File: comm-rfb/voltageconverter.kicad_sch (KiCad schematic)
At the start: 12 parts, among them Q1 Q_PMOS_DGS, U3 BU33SA5WGWZ-E2-qsat-symb

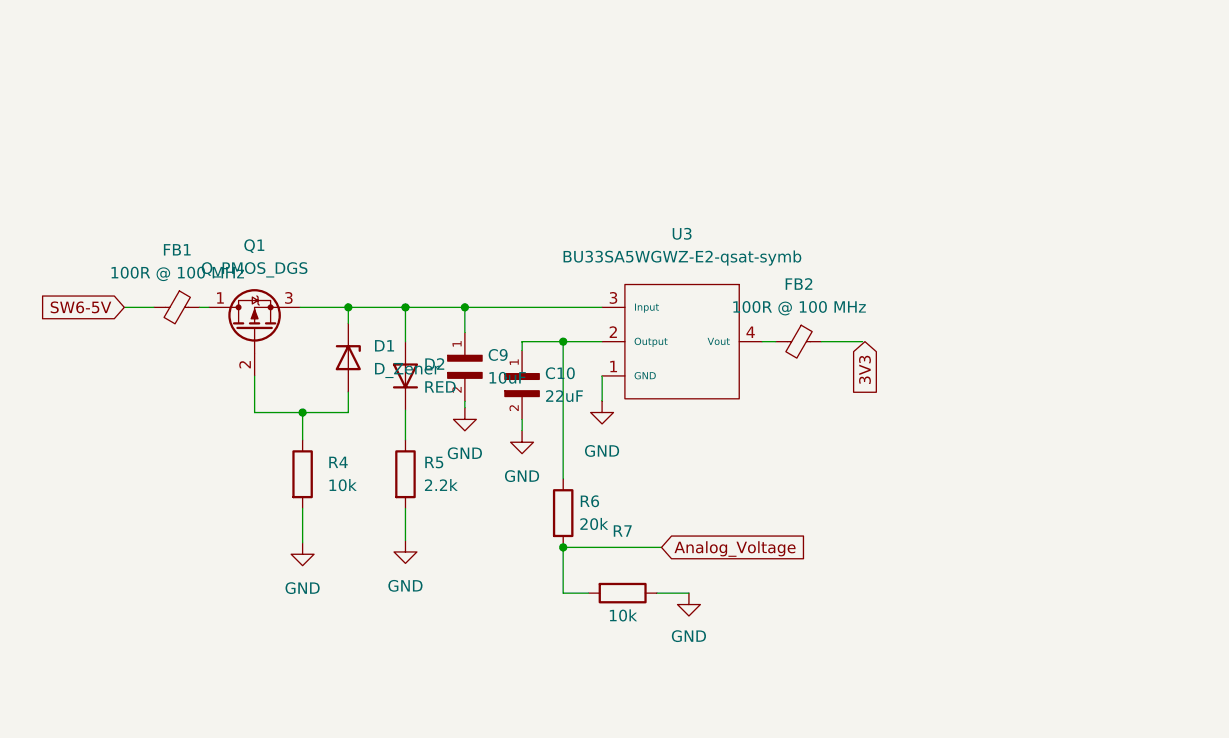
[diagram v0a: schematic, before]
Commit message: comm-rfb: reduce number of sheets in schematic
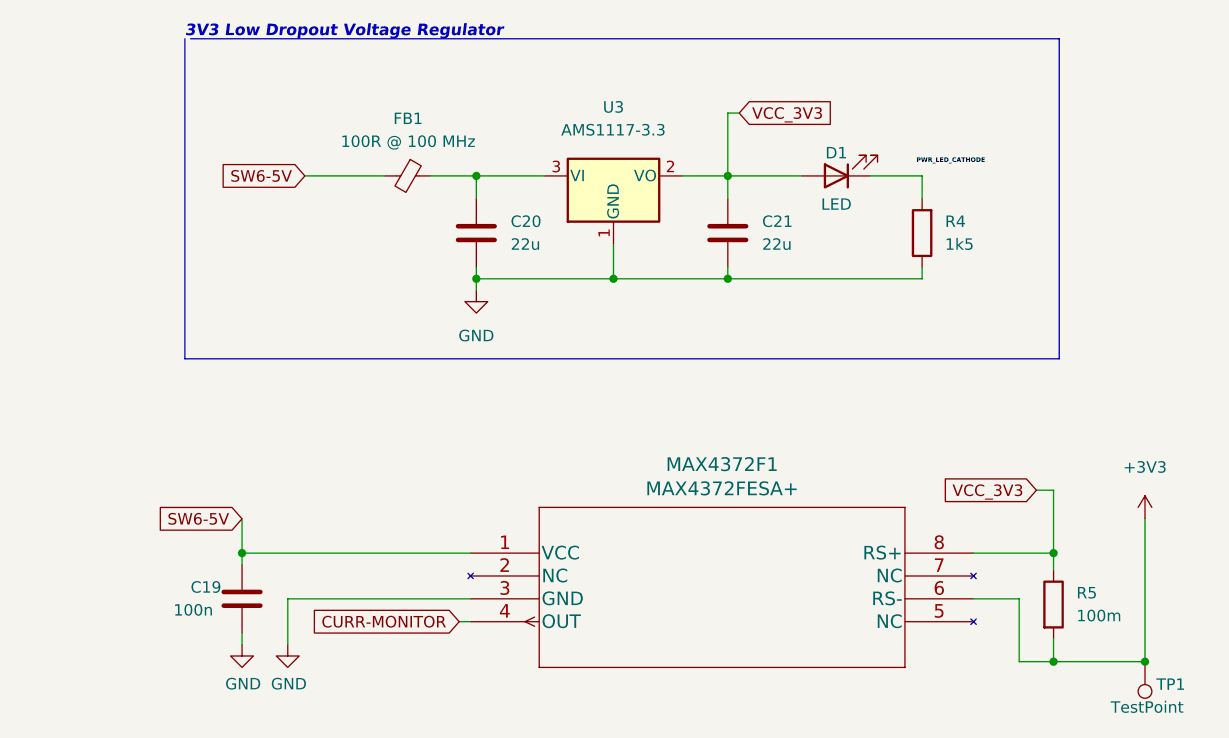
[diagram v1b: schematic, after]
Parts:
- removed C10: 22uF, CAPC1608X90N, symbol Daughterboard_Symbols:CL10B104KB8NNNL
- removed C9: 10uF, CAPC1608X90N, symbol Daughterboard_Symbols:CL10B104KB8NNNL
- removed D1: D_Zener, STM32_Breakout:SOT91P240X110-3N, symbol Device:D_Zener
- removed D2: RED, Daughterboard_footprints:CAPC1608X90N, symbol Simulation_SPICE:DIODE
- removed FB2: 100R @ 100 MHz, Daughterboard_footprints:BEADC1608X75N, symbol Device:FerriteBead_Small
- removed Q1: Q_PMOS_DGS, STM32_Breakout:SOT91P240X110-3N, symbol Device:Q_PMOS_DGS
- removed R6: 20k, Daughterboard_footprints:RESC1608X55N, symbol Device:R
- removed R7: 10k, Daughterboard_footprints:RESC1608X55N, symbol Device:R
- removed U3: BU33SA5WGWZ-E2-qsat-symb, STM32_Breakout:BU33SA5WGWZ-E2, symbol Imported_OBC_Library:BU33SA5WGWZ-E2-qsat-symb
- added C19: 100n, Capacitor_SMD:C_0603_1608Metric, symbol Device:C
- added C20, C21: 22u, Capacitor_SMD:C_0805_2012Metric, symbol Device:C
- added D1: LED, LED_SMD:LED_0603_1608Metric, symbol Device:LED
- added MAX4372F1: MAX4372FESA+, STM32_Breakout:SOIC127P600X175-8N, symbol STM32_Breakout-rescue:MAX4372FESA+-MAX4372FESA+
- added TP1: TestPoint, TestPoint:TestPoint_Pad_D2.0mm, symbol Connector:TestPoint
- added U3: AMS1117-3.3, Package_TO_SOT_SMD:SOT-223-3_TabPin2, symbol Regulator_Linear:AMS1117-3.3
- FB1: footprint Daughterboard_footprints:BEADC1608X75N -> Inductor_SMD:L_0603_1608Metric
- R4: value 10k -> 1k5; footprint Daughterboard_footprints:RESC1608X55N -> Resistor_SMD:R_0603_1608Metric
- R5: value 2.2k -> 100m; footprint Daughterboard_footprints:RESC1608X55N -> Resistor_SMD:R_0603_1608Metric
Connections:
- net GND: now also R4.1, C19.2, C20.2, C21.2, MAX4372F1.3 (GND), U3.1 (GND); no longer R4.2, R5.2
- net SW6-5V: now also C19.1, MAX4372F1.1 (VCC)
- net at FB1.1: now also C20.1, U3.3 (VI)
- net VCC_3V3: now reaches R5.1
- net VCC_3V3: now also C21.1, D1.2 (A), MAX4372F1.8 (RS+), U3.2 (VO)
- new net: D1.1 (K), R4.2
- new net +3V3: MAX4372F1.6 (RS-), R5.2, TP1.1
- new net CURR-MONITOR: MAX4372F1.4 (OUT)
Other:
- note added: "3V3 Low Dropout Voltage Regulator"
- moved on the sheet: FB1
